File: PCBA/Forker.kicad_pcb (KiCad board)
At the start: 2 copper layers, 60.5 x 51 mm, 48 parts, among them J1 USB C, J11 Conn_01x05, J12 Conn_02x06_Odd_Even, J2 Conn_01x02, J3 Conn_01x06, J4 AA, J5 AA, J6 Conn_01x02, J7 Conn_01x02, J8 Conn_01x02, J9 Conn_01x02, SW8 SPDT, U1 BQ21040, U2 RT9078, U3 MSPM0L1304, U4 XT1861, U5 HL118, U6 HL118, U7 HL118, U8 HL118

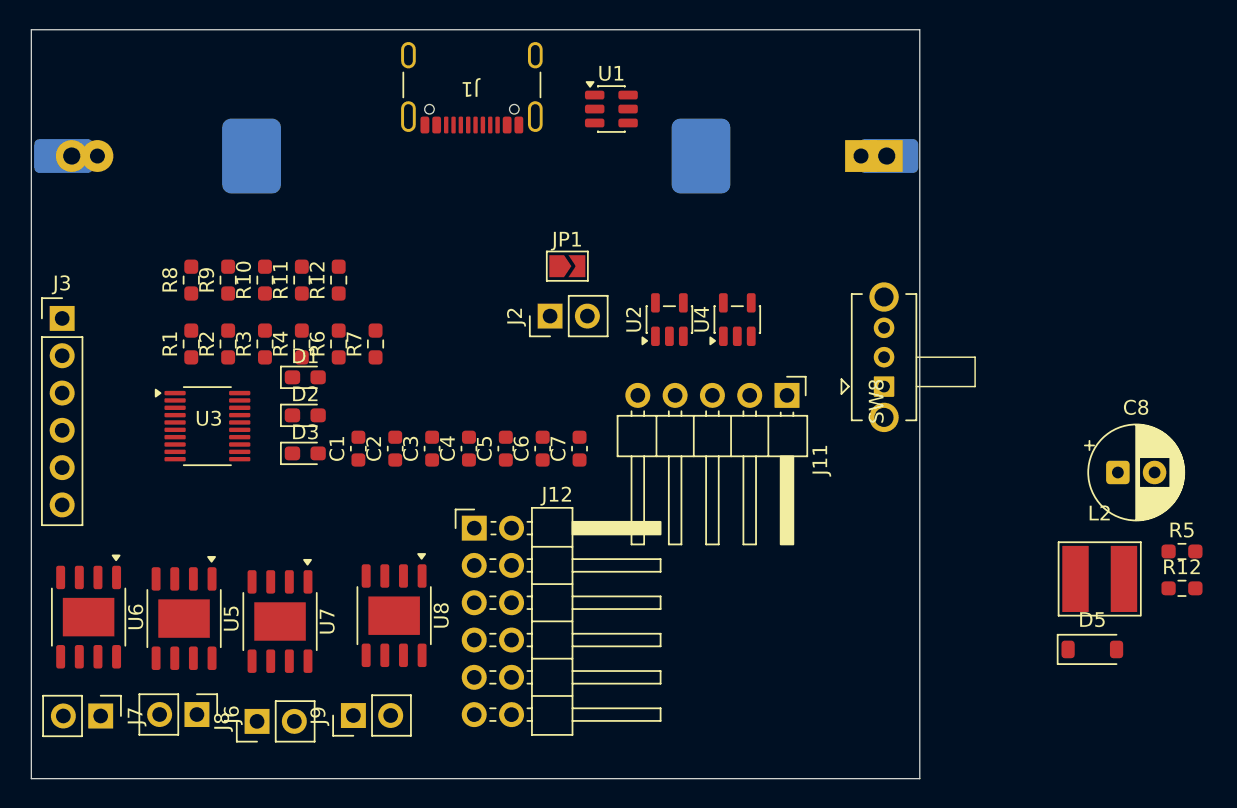
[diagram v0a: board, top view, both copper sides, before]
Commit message: Update PCB Layout
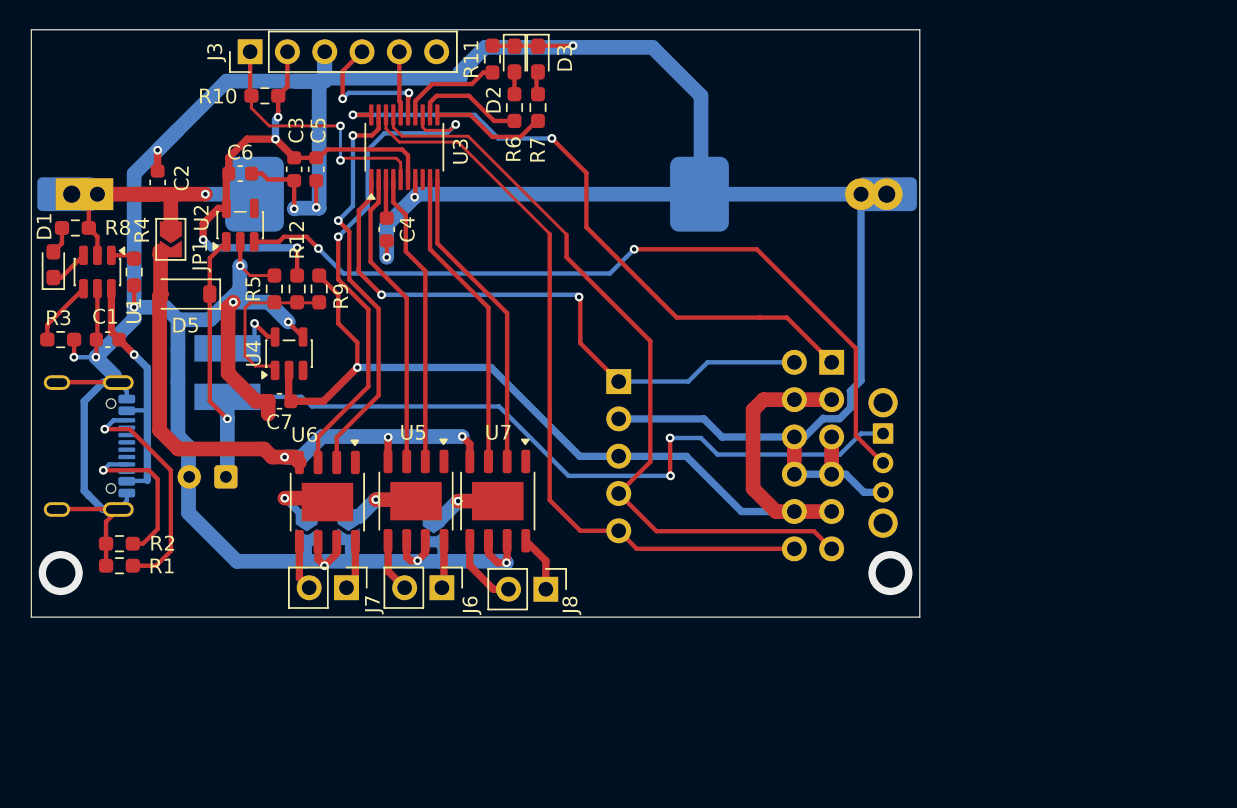
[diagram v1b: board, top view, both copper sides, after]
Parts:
- removed J2, J9: Conn_01x02, Connector_PinHeader_2.54mm:PinHeader_1x02_P2.54mm_Vertical
- removed the R12 at (120.9, 66.0)
- removed U8: HL118, Local_Footprints:SOP-8-1EP_3.9x4.9mm_P1.27mm_EP2.4x3.3mm
- added JP2: SolderJumper_2_Open, Jumper:SolderJumper-2_P1.3mm_Open_TrianglePad1.0x1.5mm, B.Cu at (121.6, 82.9)
- added JP3: SolderJumper_2_Open, Jumper:SolderJumper-2_P1.3mm_Open_TrianglePad1.0x1.5mm, B.Cu at (118.8, 82.9)
- added JP4: SolderJumper_2_Open, Jumper:SolderJumper-2_P1.3mm_Open_TrianglePad1.0x1.5mm, B.Cu at (127.4, 83.0)
- C8, J1, J11, J12, L2, SW8: moved to B.Cu
- moved D5 66.3 mm to (110.5, 67.0), turned to 180 degrees
- moved R5 64.3 mm to (116.5, 66.7), turned to 90 degrees
- moved R12 63.6 mm to (118.1, 66.7), turned to 90 degrees
- moved L2 61.0 mm to (113.3, 72.3), turned to 90 degrees
- moved C8 60.7 mm to (113.2, 79.5), turned to 180 degrees
- moved U1 36.7 mm to (104.5, 65.5), turned to -90 degrees
- moved J1 36.0 mm to (103.7, 77.3), turned to 90 degrees
- moved D3 31.2 mm to (134.5, 51.0), turned to -90 degrees
- moved U4 30.6 mm to (117.5, 71.1)
- moved U2 29.9 mm to (114.2, 62.3)
- moved D2 28.1 mm to (132.9, 51.0), turned to -90 degrees
- moved C6 27.8 mm to (114.2, 58.8), turned to 0 degrees
- moved JP1 27.1 mm to (109.5, 63.3), turned to -90 degrees
- moved J12 26.8 mm to (154.5, 71.7), turned to 180 degrees
- moved C2 24.3 mm to (108.6, 59.4)
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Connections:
- R4 pad 1: unconnected-(R4-Pad1) -> GND
- R4 pad 2: unconnected-(R4-Pad2) -> Net-(U1-TS)
- U1 pad 1: unconnected-(U1-TS-Pad1) -> Net-(U1-TS)
- U3 pad 8: Net-(U3-PA2/ROSC) -> unconnected-(U3-PA2/ROSC-Pad8)
- U5 pad 1: (no net) -> unconnected-(U5-NC-Pad1)
- U5 pad 9: (no net) -> Net-(JP2-A)
- U6 pad 1: (no net) -> unconnected-(U6-NC-Pad1)
- U6 pad 3: Net-(U3-PA18/A7/BSL) -> Net-(U3-PA17)
- U6 pad 9: (no net) -> Net-(JP3-A)
- U7 pad 1: (no net) -> unconnected-(U7-NC-Pad1)
- U7 pad 2: Net-(U3-PA17) -> Net-(U3-PA6)
- U7 pad 3: Net-(U3-PA6) -> Net-(U3-PA4)
- U7 pad 9: (no net) -> Net-(JP4-A)
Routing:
- net GND: track 0.00 -> 300.6 mm, vias 0 -> 15
- net Net-(D5-K): track 0.00 -> 69.1 mm, vias 0 -> 3
- net +5V: track 0.00 -> 65.8 mm, vias 0 -> 1
- net Net-(U2-EN): track 0.00 -> 54.2 mm, vias 0 -> 2
- net /RADIO_TX: track 0.00 -> 52.6 mm
- net /RADIO_RX: track 0.00 -> 51.2 mm
- net Net-(J12-Pin_1): track 0.00 -> 43.0 mm, vias 0 -> 2
- net /RADIO_BOOT: track 0.00 -> 41.8 mm, vias 0 -> 2
- net +BATT: track 0.00 -> 39.0 mm, vias 0 -> 3
- net +3V3: track 0.00 -> 36.8 mm, vias 0 -> 4
- net Net-(U3-PA17): track 0.00 -> 34.4 mm, vias 0 -> 2
- net Net-(U3-PA24/A3): track 0.00 -> 27.9 mm, vias 0 -> 2
- net Net-(U3-PA6): track 0.00 -> 21.2 mm
- net Net-(U3-PA4): track 0.00 -> 20.8 mm
- net Net-(U3-PA27/A0): track 0.00 -> 20.4 mm
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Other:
- board size 60.5 x 51 mm -> 60.5 x 40 mm
